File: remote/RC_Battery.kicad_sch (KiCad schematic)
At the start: 18 parts, among them P1 JST CONN, SW3 YTSPS-22E58LM, U2 MCP73831-5-OT, U3 AP62300Z6

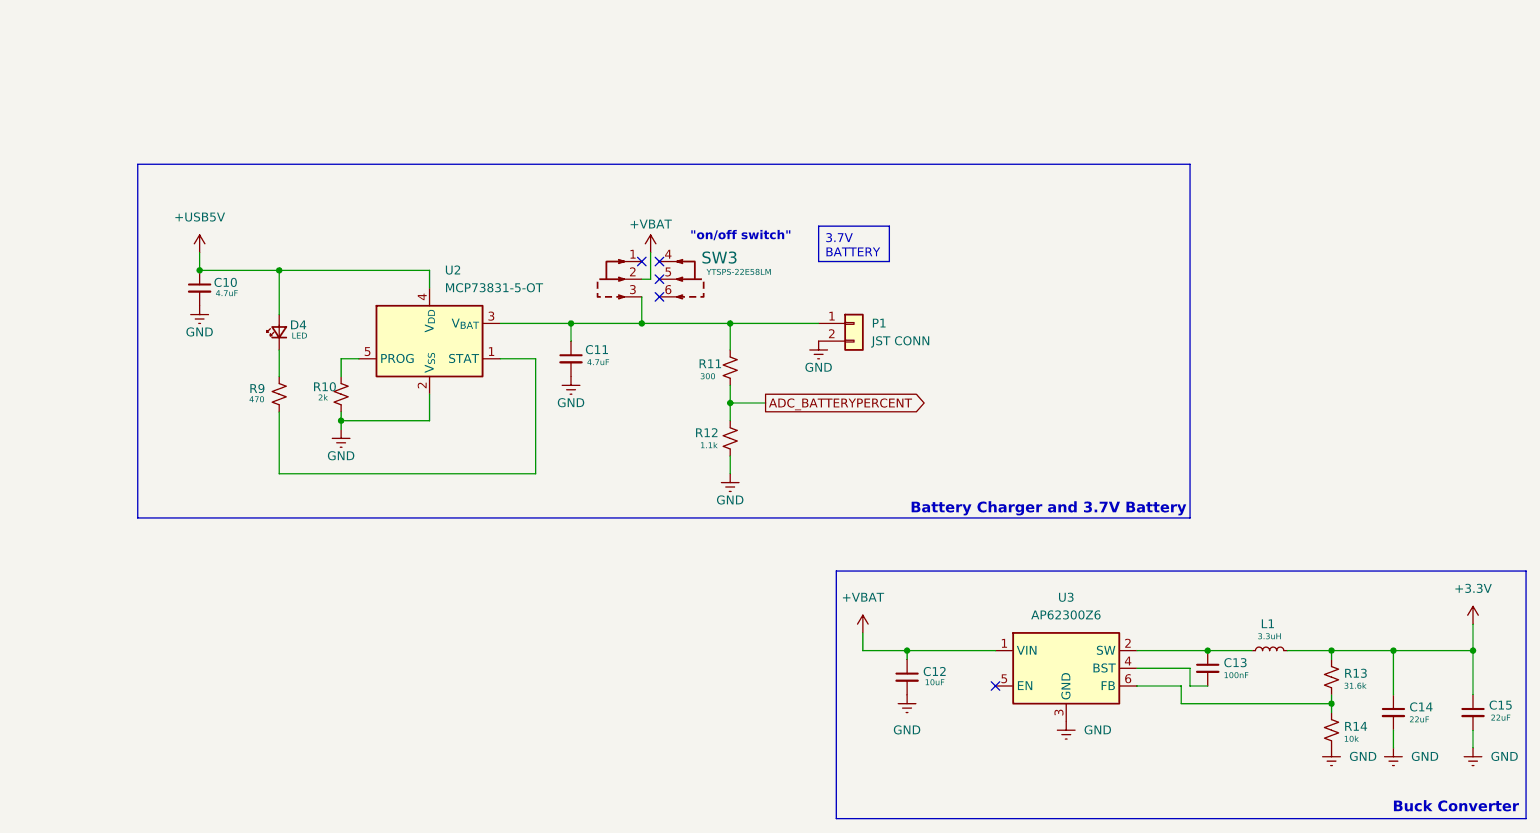
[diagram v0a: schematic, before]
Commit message: CRC V3
V 3.0.0
Initial version of CRC V3, fully redesigned remote
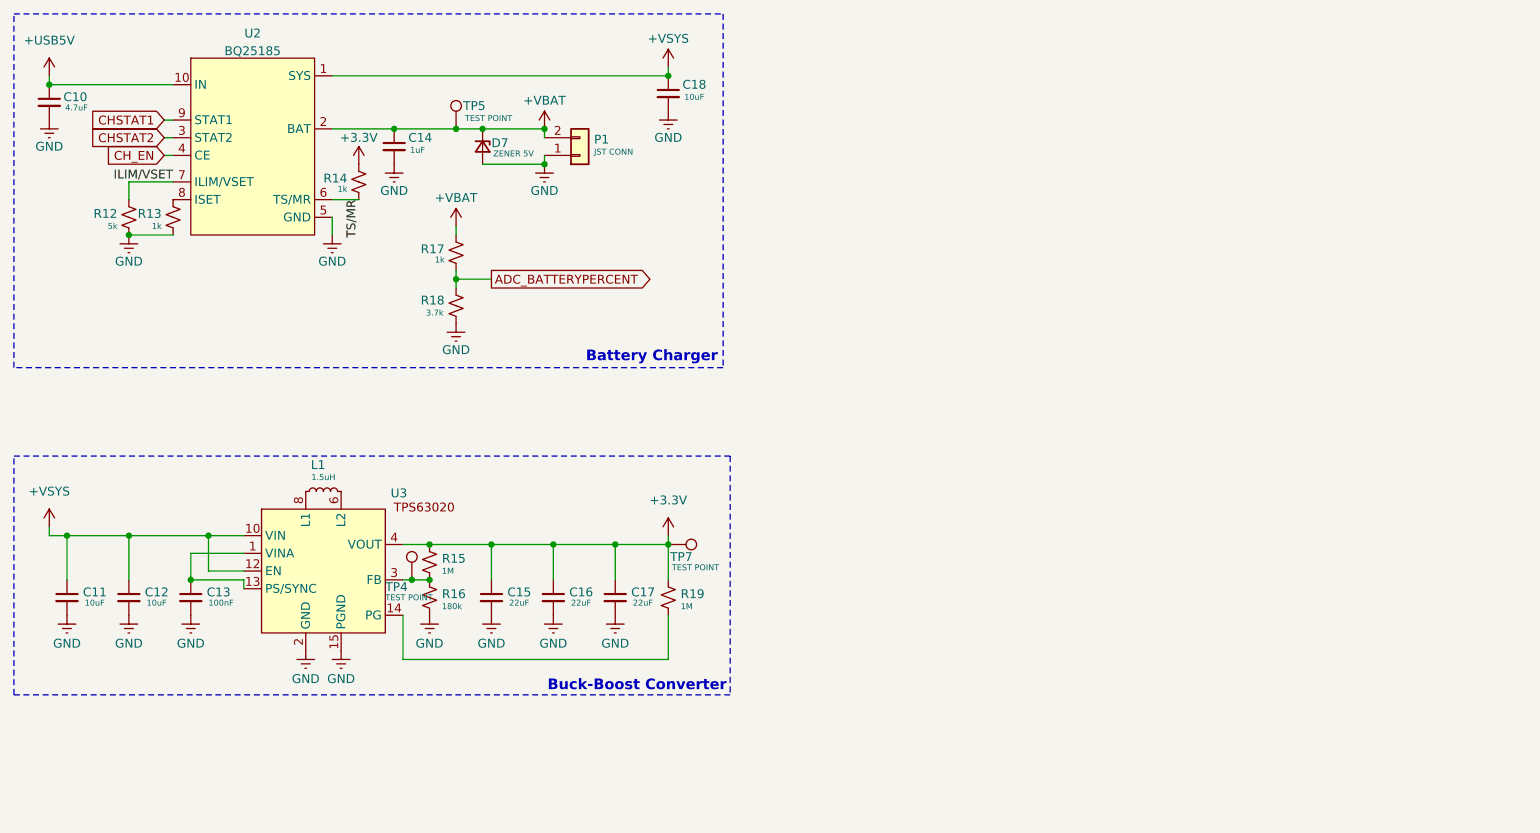
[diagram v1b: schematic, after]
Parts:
- removed C11: 4.7uF, Capacitor_SMD:C_0402_1005Metric, symbol Device:C_Small
- removed D4: LED, footprints:D_0402_1005Metric, symbol Device:LED_Small
- removed R10: 2k, Resistor_SMD:R_0402_1005Metric, symbol Device:R_Small_US
- removed R11: 300, Resistor_SMD:R_0402_1005Metric, symbol Device:R_Small_US
- removed R9: 470, Resistor_SMD:R_0402_1005Metric, symbol Device:R_Small_US
- removed SW3: YTSPS-22E58LM, footprints:SW-SMD_6P-YTSPS-22E58LM, symbol components:YTSPS-22E58LM
- removed U2: MCP73831-5-OT, Package_DFN_QFN:DFN-8-1EP_2x3mm_P0.5mm_EP0.61x2.2mm, symbol Battery_Management:MCP73831-5-OT
- removed U3: AP62300Z6, Package_TO_SOT_SMD:SOT-563, symbol Regulator_Switching:AP62300Z6
- added C12: 10uF, Capacitor_SMD:C_0603_1608Metric_Pad1.08x0.95mm_HandSolder, symbol Device:C_Small
- added C16, C17: 22uF, Capacitor_SMD:C_0603_1608Metric_Pad1.08x0.95mm_HandSolder, symbol Device:C_Small
- added C18: 10uF, Capacitor_SMD:C_0402_1005Metric_Pad0.74x0.62mm_HandSolder, symbol Device:C_Small
- added D7: ZENER 5V, Diode_SMD:D_0402_1005Metric_Pad0.77x0.64mm_HandSolder, symbol Device:D_Zener_Small
- added R13, R17: 1k, Resistor_SMD:R_0402_1005Metric_Pad0.72x0.64mm_HandSolder, symbol Device:R_Small_US
- added R16: 180k, Resistor_SMD:R_0402_1005Metric_Pad0.72x0.64mm_HandSolder, symbol Device:R_Small_US
- added R18: 3.7k, Resistor_SMD:R_0402_1005Metric_Pad0.72x0.64mm_HandSolder, symbol Device:R_Small_US
- added R19: 1M, Resistor_SMD:R_0402_1005Metric_Pad0.72x0.64mm_HandSolder, symbol Device:R_Small_US
- added TP4, TP5, TP7: TEST POINT, TestPoint:TestPoint_Pad_2.0x2.0mm, symbol Connector:TestPoint
- added U2: BQ25185, footprints:WSON-10 BQ25185, symbol components:BQ25185
- added U3: TPS63020, footprints:TPS63020_VSON(14), symbol components:TPS63020
- C10: footprint Capacitor_SMD:C_0402_1005Metric -> Capacitor_SMD:C_0402_1005Metric_Pad0.74x0.62mm_HandSolder
- C11: renamed from C12; footprint Capacitor_SMD:C_0603_1608Metric -> Capacitor_SMD:C_0603_1608Metric_Pad1.08x0.95mm_HandSolder
- C13: footprint Capacitor_SMD:C_0402_1005Metric -> Capacitor_SMD:C_0603_1608Metric_Pad1.08x0.95mm_HandSolder; LCSC# C1525 -> C95839; MPN C1525 -> C95839
- C14: value 22uF -> 1uF; footprint Capacitor_SMD:C_0805_2012Metric -> Capacitor_SMD:C_0402_1005Metric_Pad0.74x0.62mm_HandSolder; LCSC# C87997 -> C23733; MPN C87997 -> C23733
- C15: footprint Capacitor_SMD:C_0805_2012Metric -> Capacitor_SMD:C_0603_1608Metric_Pad1.08x0.95mm_HandSolder; LCSC# C87997 -> C95839; MPN C87997 -> C95839
- L1: value 3.3uH -> 1.5uH
- R12: value 1.1k -> 5k; footprint Resistor_SMD:R_0402_1005Metric -> Resistor_SMD:R_0402_1005Metric_Pad0.72x0.64mm_HandSolder; LCSC# C445597 -> C852712; MPN C445597 -> C852712
- R14: value 10k -> 1k; footprint Resistor_SMD:R_0402_1005Metric -> Resistor_SMD:R_0402_1005Metric_Pad0.72x0.64mm_HandSolder; LCSC# C190095 -> C852712; MPN C190095 -> C852712
- R15: renamed from R13; value 31.6k -> 1M; footprint Resistor_SMD:R_0402_1005Metric -> Resistor_SMD:R_0402_1005Metric_Pad0.72x0.64mm_HandSolder
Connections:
- net +3.3V: now also R14.1, C16.1, C17.1, R19.1, TP7.1, U3.4 (VOUT), U3.5 (VOUT); no longer C14.1, L1.2
- net +USB5V: now also U2.10 (IN)
- net +VBAT: now also C14.1, P1.2 (Pin_2), D7.1 (K), R17.1, TP5.1, U2.2 (BAT); no longer C11.1
- net ADC_BATTERYPERCENT: now also R17.2, R18.1; no longer R12.1
- net GND: now also C13.2, P1.1 (Pin_1), C12.2, C16.2, C17.2, C18.2, D7.2 (A), R13.2, R16.2, R18.2, U2.5 (GND), U3.15 (PGND), U3.2 (GND); no longer P1.2 (Pin_2), R14.2
- net at L1.1: now also U3.8 (L1), U3.9 (L1); no longer C13.1
- net at R15.2: now also R16.1, TP4.1, U3.3 (FB); no longer R14.1
- new net: R13.1, U2.8 (ISET)
- new net: L1.2, U3.6 (L2), U3.7 (L2)
- new net: R19.2, U3.14 (PG)
- new net: C13.1, U3.1 (VINA), U3.13 (PS/SYNC)
- new net +VSYS: C11.1, C12.1, C18.1, U2.1 (SYS), U3.10 (VIN), U3.11 (VIN), U3.12 (EN)
- new net CHSTAT1: U2.9 (STAT1)
- new net CHSTAT2: U2.3 (STAT2)
- new net CH_EN: U2.4 (CE)
- new net ILIM/VSET: R12.1, U2.7 (ILIM/VSET)
- new net TS/MR: R14.2, U2.6 (TS/MR)
- no-connect marks 5 -> 0
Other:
- note added: "Battery Charger"
- note added: "Buck-Boost Converter"
- note removed: "Battery Charger and 3.7V Battery"
- note removed: "Buck Converter"
- note removed: "{dblquote}on/off switch{dblquote}"
- moved on the sheet: C11, L1, R15
